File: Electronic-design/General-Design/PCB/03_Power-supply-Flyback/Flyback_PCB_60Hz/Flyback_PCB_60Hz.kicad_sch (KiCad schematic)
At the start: 1 part, among them J1 4300.0104

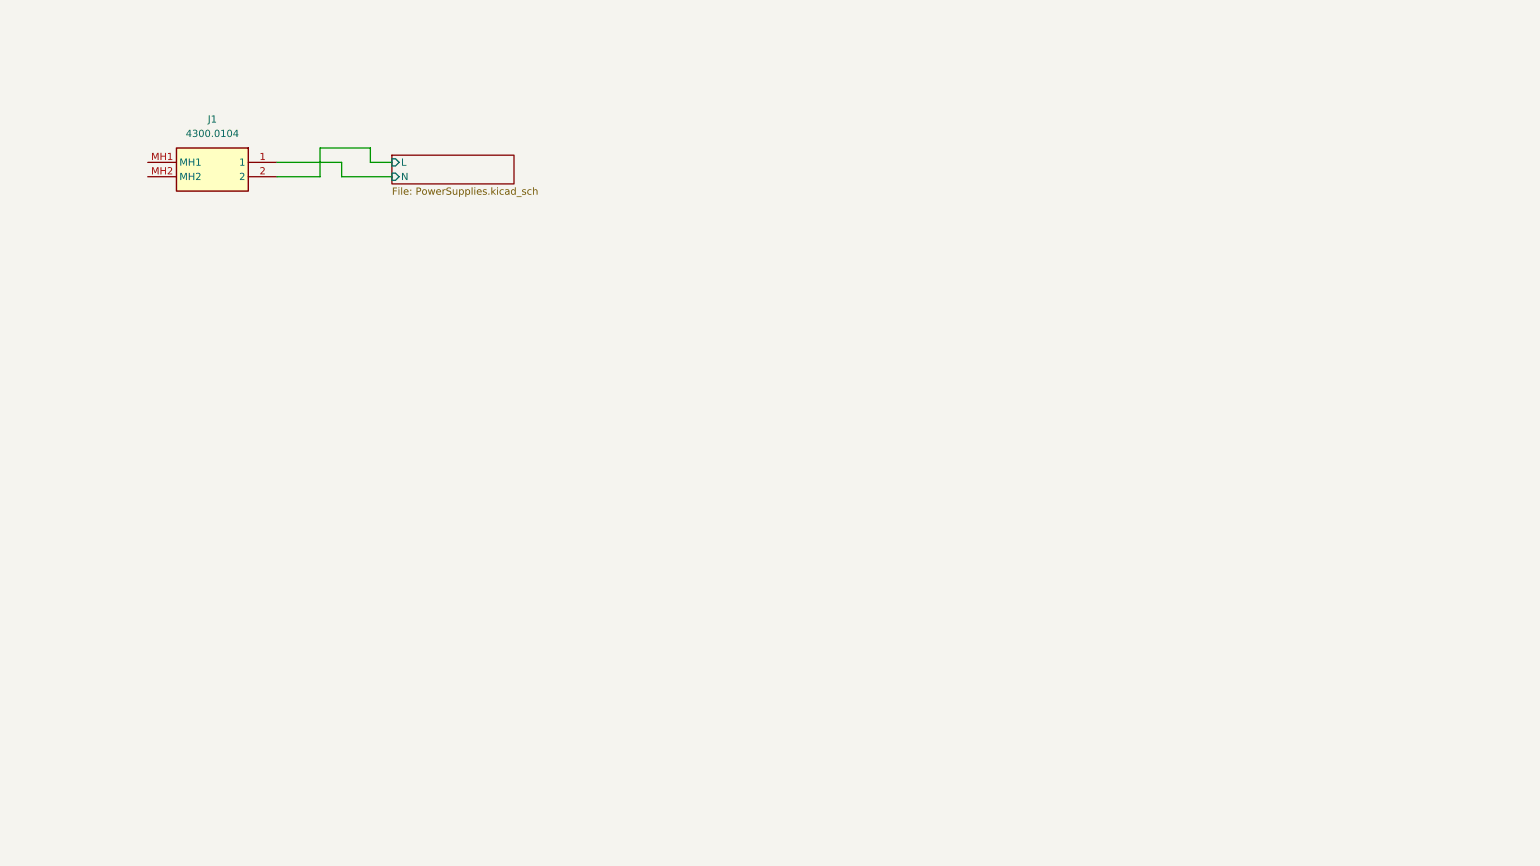
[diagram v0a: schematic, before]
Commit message: Flyback-onto-03-V1
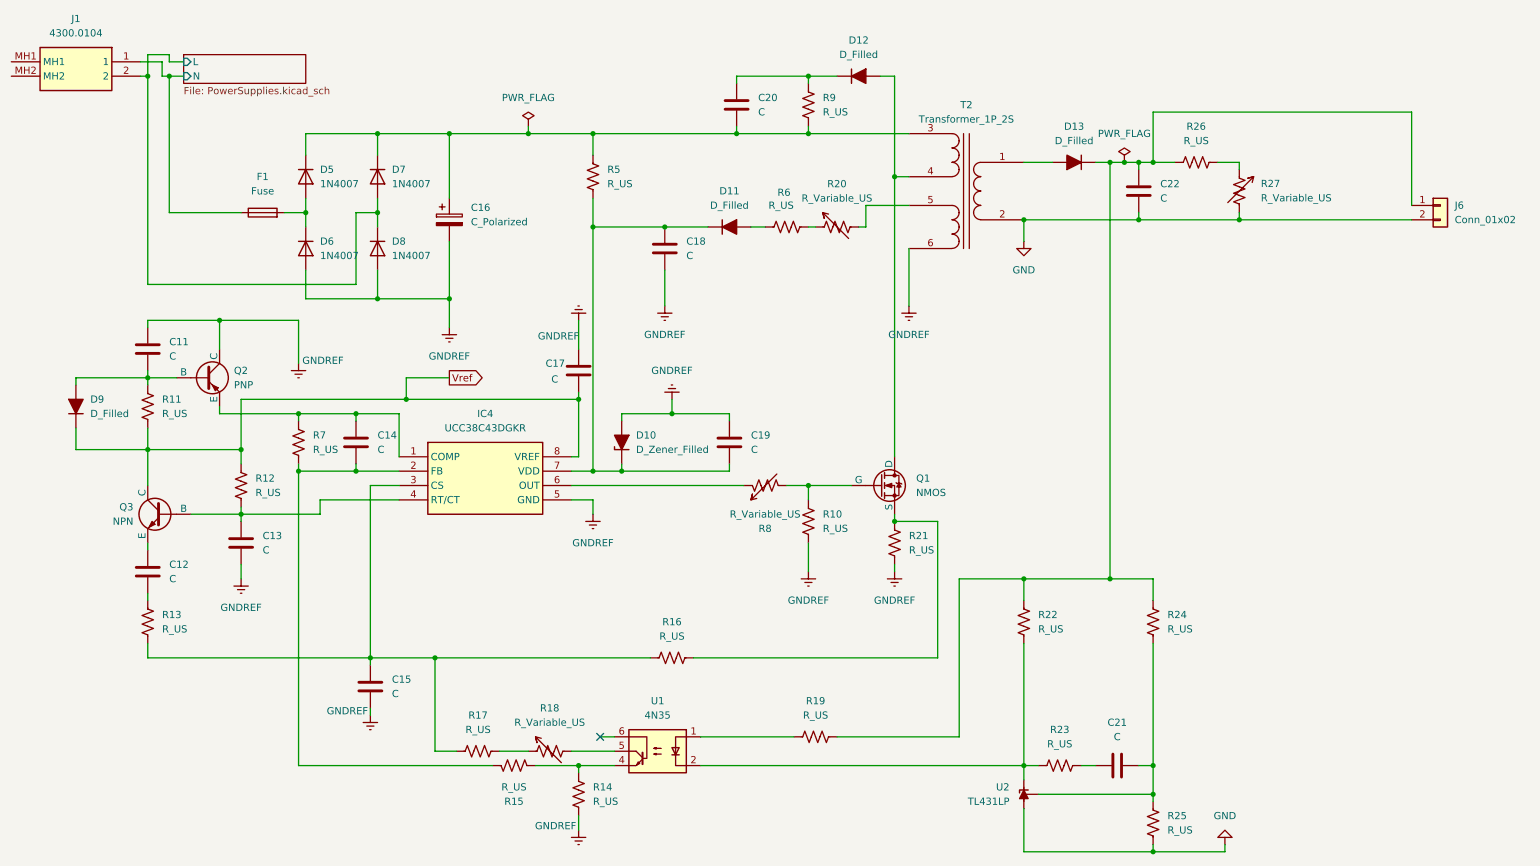
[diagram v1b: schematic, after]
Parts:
- added C11, C12, C13, C14, C15, C17, C18, C19, C20, C21, C22: C, symbol Device:C
- added C16: C_Polarized, symbol Device:C_Polarized
- added D10: D_Zener_Filled, symbol Device:D_Zener_Filled
- added D11, D12, D13, D9: D_Filled, symbol Device:D_Filled
- added D5, D6, D7, D8: 1N4007, Diode_THT:D_DO-41_SOD81_P10.16mm_Horizontal, symbol Diode:1N4007
- added F1: Fuse, symbol Device:Fuse
- added IC4: UCC38C43DGKR, Footprints:SOP65P490X110-8N, symbol UCC38C43DGKR:UCC38C43DGKR
- added J6: Conn_01x02, Connector_JST:JST_XH_B2B-XH-A_1x02_P2.50mm_Vertical, symbol Connector_Generic:Conn_01x02
- added Q1: NMOS, symbol Simulation_SPICE:NMOS
- added Q2: PNP, symbol Simulation_SPICE:PNP
- added Q3: NPN, symbol Simulation_SPICE:NPN
- added R10, R11, R12, R13, R14, R15, R16, R17, R19, R21, R22, R23, R24, R25, R26, R5, R6, R7, R9: R_US, symbol Device:R_US
- added R18, R20, R27, R8: R_Variable_US, symbol Device:R_Variable_US
- added T2: Transformer_1P_2S, symbol Device:Transformer_1P_2S
- added U1: 4N35, Package_DIP:DIP-6_W7.62mm, symbol Isolator:4N35
- added U2: TL431LP, Package_TO_SOT_THT:TO-92_Inline, symbol Reference_Voltage:TL431LP
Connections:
- net Supplies/L: now also D7.2 (A), D8.1 (K)
- net Supplies/N: now also F1.1
- new net: D11.2 (A), R6.1
- new net: R20.1, R6.2
- new net: C21.1, R23.1
- new net: C21.2, R24.2, R25.1, U2.1 (REF)
- new net: C22.1, D13.1 (K), J6.1 (Pin_1), R19.1, R22.1, R24.1, R26.1
- new net: D13.2 (A), T2.1 (AA)
- new net: C11.2, D9.2 (A), Q2.2 (B), R11.1
- new net: C14.1, IC4.1 (COMP), Q2.3 (E), R7.1
- new net: C14.2, IC4.2 (FB), R15.1, R7.2
- new net: D5.2 (A), D6.1 (K), F1.2
- new net: C20.1, D12.1 (K), R9.1
- new net: C16.1, C20.2, D5.1 (K), D7.1 (K), R5.1, R9.2, T2.3 (SA)
- new net: C18.1, C19.2, D10.1 (K), D11.1 (K), IC4.7 (VDD), R5.2
- new net: C12.2, R13.1
- new net: C15.1, IC4.3 (CS), R13.2, R16.1, R17.1
- new net: R17.2, R18.1
- new net: D12.2 (A), Q1.1 (D), T2.4 (SB)
- new net: R26.2, R27.1
- new net: C13.1, IC4.4 (RT/CT), Q3.2 (B), R12.2
- new net: IC4.6 (OUT), R8.1
- new net: C12.1, Q3.3 (E)
- new net: Q1.2 (G), R10.1, R8.2
- new net: R18.2, U1.5
- new net: R19.2, U1.1
- new net: R22.2, R23.2, U1.2, U2.3 (K)
- new net: R14.1, R15.2, U1.4
- new net: Q1.3 (S), R16.2, R21.1
- new net: R20.2, T2.5 (SC)
- new net GND: C22.2, J6.2 (Pin_2), R25.2, R27.2, T2.2 (AB), U2.2 (A)
- new net GNDREF: C11.1, C13.2, C15.2, C16.2, C17.1, C18.2, C19.1, D10.2 (A), D6.2 (A), D8.2 (A), IC4.5 (GND), Q2.1 (C), R10.2, R14.2, R21.2, T2.6 (SD)
- new net Vref: C17.2, D9.1 (K), IC4.8 (VREF), Q3.1 (C), R11.2, R12.1
- no-connect marks 0 -> 1
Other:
- moved on the sheet: J1
